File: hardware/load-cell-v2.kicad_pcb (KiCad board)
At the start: 2 copper layers, 30 x 30 mm, 36 parts, among them P1 CON-SENSOR, P2 Boot, P3 Debug, P4 AKL_5_2, P5 AKL_5_2, U1 XMC1100, U2 FAN4860, U3 HX711, U4 DRILL, U5 DRILL, U6 DRILL, U7 DRILL

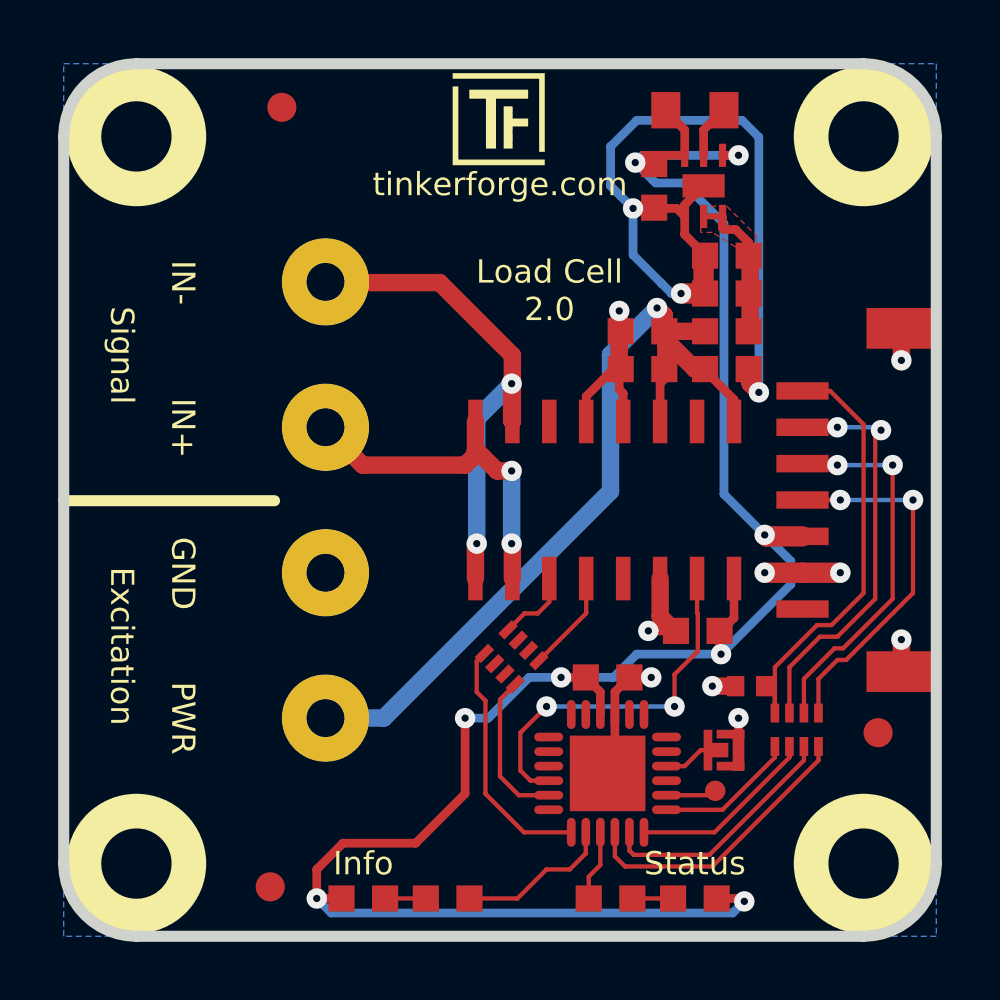
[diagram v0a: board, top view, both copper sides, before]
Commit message: move to new kicad version
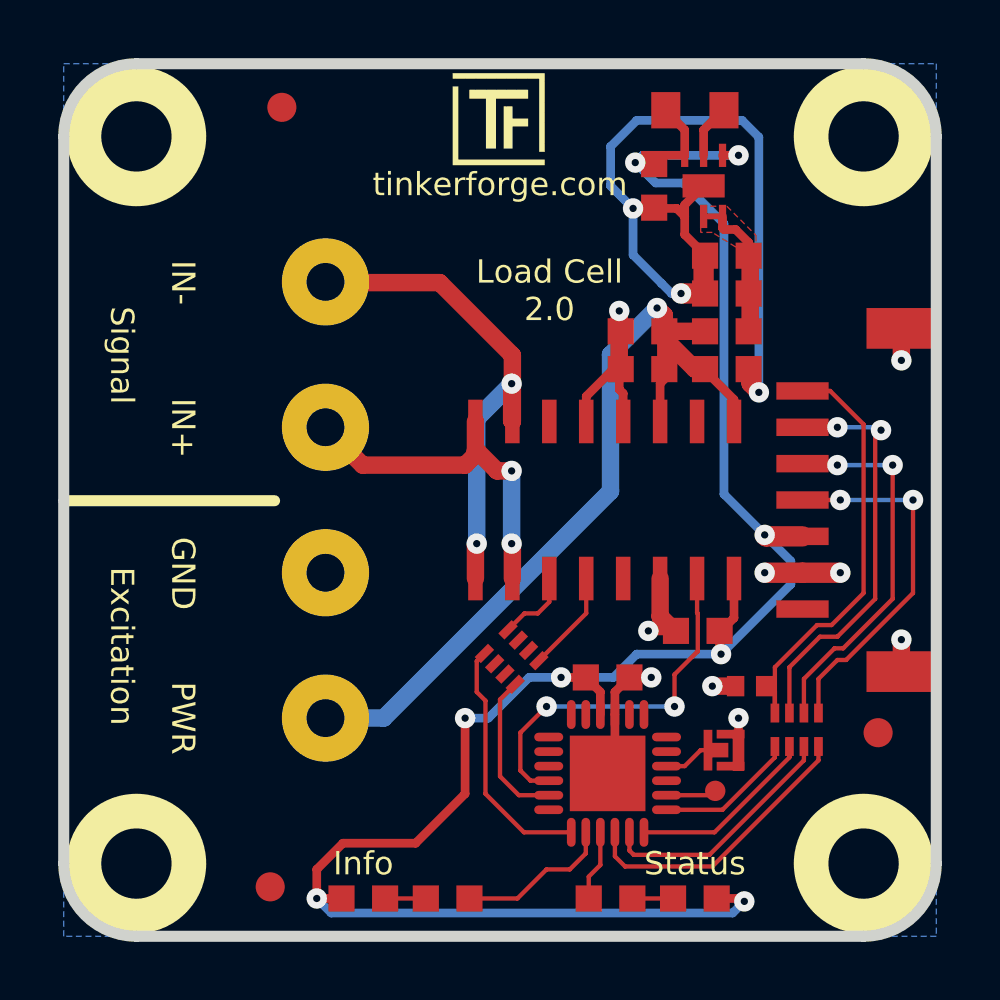
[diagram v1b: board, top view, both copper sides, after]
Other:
- net class Default removed
